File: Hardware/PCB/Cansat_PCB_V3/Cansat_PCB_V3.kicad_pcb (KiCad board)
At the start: 6 copper layers, 33.6 x 25.4 mm, 100 parts, among them IC1 Alim STM Baro GPS IMU, IC2 Alim LoRa, J1 Lecteur SD, J10 Connecteur IHM, J2 Connecteur Batterie, J3 Connecteur STLINK, J4 Connecteur Moteur, J5 Connecteur TOF, J6 Connecteur GPS, J7 Connecteur LoRa, J9 Connecteur Camera, SW1 RSTBTN, SW2 boot, U1 Barometre BMP581, U2 STM32G431CBUx, U3 IMU BNO055, U5 LMR51625, Y1 Crystal_GND24_Small, Y2 Oscillateur_IMU

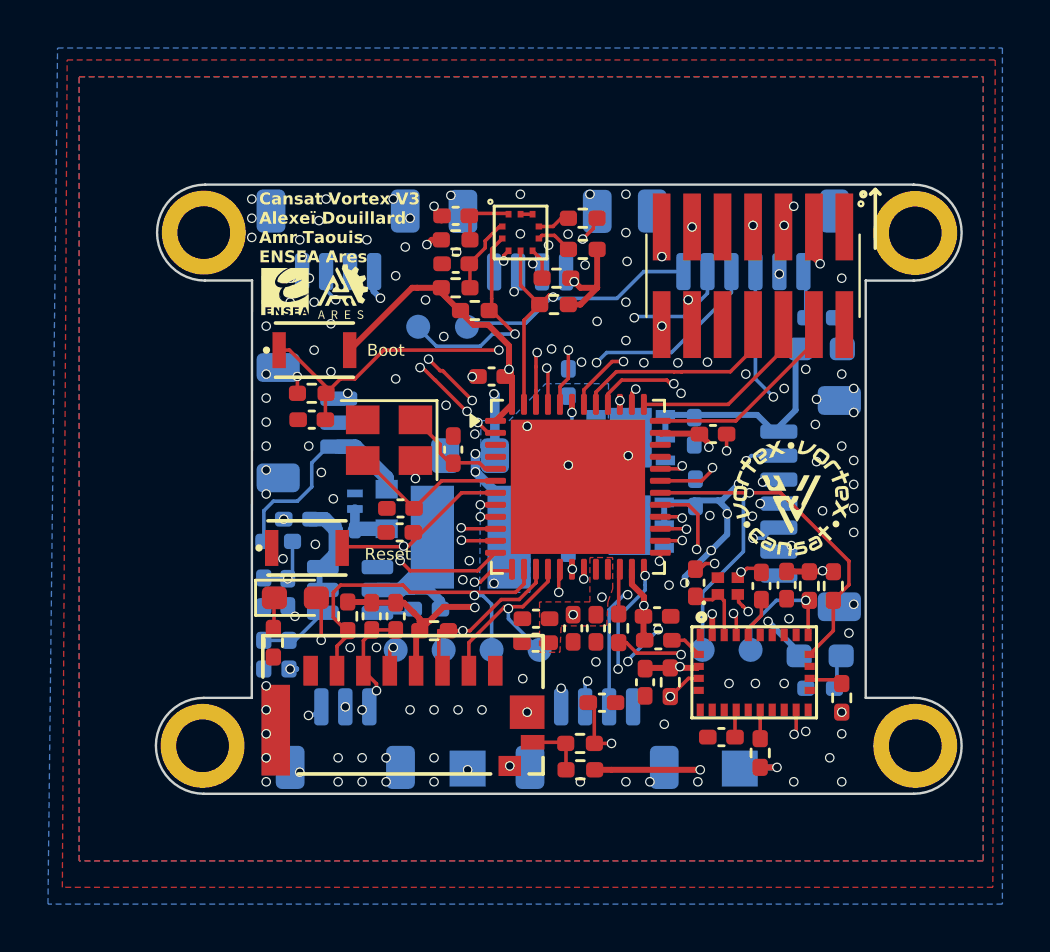
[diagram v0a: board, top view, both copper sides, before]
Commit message: mega big readme update for the mechanical and wind tunnel parts
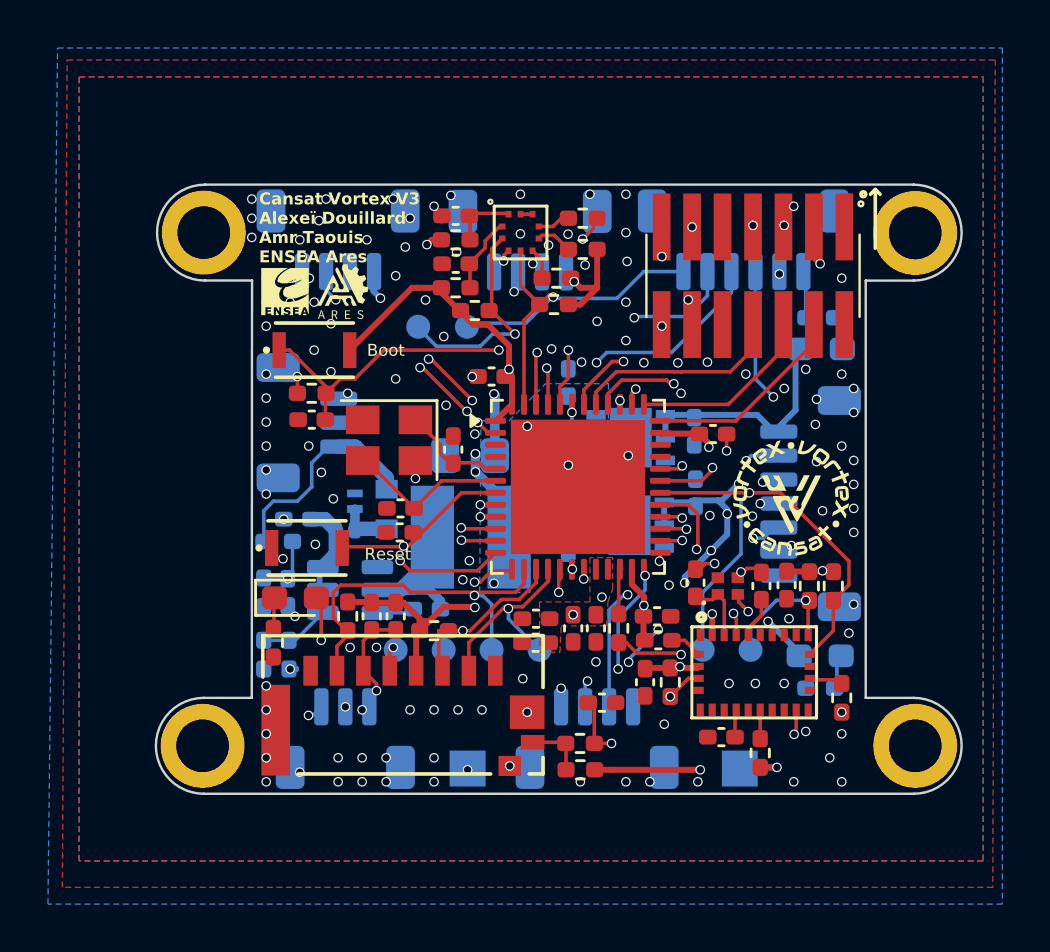
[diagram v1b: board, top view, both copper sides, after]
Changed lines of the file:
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@@
 			(drillshape 0)
 			(scaleselection 1)
-			(outputdirectory "/home/alexei/Bureau/Gerber_Cansat/")
+			(outputdirectory "/home/alexei/Bureau/Gerber_Cansat_V3/")
 		)
 	)
@@
 	)
 	(segment
-		(start 144.356471 95.85646)
-		(end 144.4 95.899989)
-		(width 0.15)
-		(layer "F.Cu")
-		(net 24)
-	)
-	(segment
-		(start 145.59 97.09)
-		(end 145.59 97.1)
+		(start 143.7716 95.375)
+		(end 143.875011 95.375)
 		(width 0.15)
 		(layer "F.Cu")
@@
 	)
 	(segment
-		(start 144.25306 95.85646)
-		(end 144.356471 95.85646)
+		(start 144.4 95.9)
+		(end 145.59 97.09)
 		(width 0.15)
 		(layer "F.Cu")
@@
 	)
 	(segment
-		(start 143.7716 95.375)
-		(end 144.25306 95.85646)
+		(start 143.875011 95.375)
+		(end 144.4 95.899989)
 		(width 0.15)
 		(layer "F.Cu")
@@
 	)
 	(segment
-		(start 144.4 95.9)
-		(end 145.59 97.09)
+		(start 144.4 95.899989)
+		(end 144.4 95.9)
 		(width 0.15)
 		(layer "F.Cu")
@@
 	)
 	(segment
-		(start 144.4 95.899989)
-		(end 144.4 95.9)
+		(start 145.59 97.09)
+		(end 145.59 97.1)
 		(width 0.15)
 		(layer "F.Cu")
@@
 	)
 	(segment
-		(start 143.4154 95.7278)
-		(end 143.520693 95.7278)
+		(start 143.520693 95.7278)
+		(end 145.344534 97.551641)
 		(width 0.15)
 		(layer "F.Cu")
@@
 	)
 	(segment
-		(start 144.059956 96.259956)
-		(end 145.351641 97.551641)
-		(width 0.15)
-		(layer "F.Cu")
-		(net 25)
-	)
-	(segment
 		(start 149.25 96.525)
 		(end 149.25 97.2625)
@@
 	)
 	(segment
-		(start 144.052849 96.259956)
-		(end 144.059956 96.259956)
+		(start 149.6 95)
+		(end 149.6 96.175)
 		(width 0.15)
 		(layer "F.Cu")
@@
 	)
 	(segment
-		(start 145.351641 97.551641)
+		(start 145.344534 97.551641)
 		(end 145.37547 97.551641)
 		(width 0.15)
@@
 	)
 	(segment
-		(start 149.6 95)
-		(end 149.6 96.175)
+		(start 143.4154 95.7278)
+		(end 143.520693 95.7278)
 		(width 0.15)
 		(layer "F.Cu")
@@
 		(net 25)
 	)
-	(segment
-		(start 143.520693 95.7278)
-		(end 144.052849 96.259956)
-		(width 0.15)
-		(layer "F.Cu")
-		(net 25)
-	)
 	(via
 		(at 149.6 95)
@@
 	)
 	(segment
-		(start 155.4 92.630043)
+		(start 155.4 92.7348)
 		(end 155.4 91.825)
 		(width 0.15)
@@
 	)
 	(segment
-		(start 154.430043 93.6)
-		(end 155.4 92.630043)
+		(start 154.5348 93.6)
+		(end 155.4 92.7348)
 		(width 0.15)
 		(layer "B.Cu")
@@
 	)
 	(segment
-		(start 152.35 93.65)
-		(end 152.4 93.6)
+		(start 147.375 94.330262)
+		(end 146.438538 94.330262)
 		(width 0.15)
 		(layer "B.Cu")
@@
 	)
 	(segment
-		(start 147.375 94.330262)
-		(end 146.438538 94.330262)
+		(start 152.4 93.6)
+		(end 154.5348 93.6)
 		(width 0.15)
 		(layer "B.Cu")
@@
 	)
 	(segment
-		(start 152.4 93.6)
-		(end 154.430043 93.6)
+		(start 152.35 93.65)
+		(end 152.4 93.6)
 		(width 0.15)
 		(layer "B.Cu")
@@
 	)
 	(via
-		(at 152.084834 107.984834)
+		(at 152.112507 108.011093)
 		(size 0.4)
 		(drill 0.3)
@@
 	)
 	(segment
-		(start 152.084834 107.922835)
-		(end 153.35 106.657669)
+		(start 152.084834 107.98342)
+		(end 152.084834 107.922835)
 		(width 0.15)
 		(layer "B.Cu")
@@
 	)
 	(segment
-		(start 152.084834 107.984834)
-		(end 152.084834 107.922835)
+		(start 152.084834 107.922835)
+		(end 153.35 106.657669)
 		(width 0.15)
 		(layer "B.Cu")
@@
 	)
 	(segment
-		(start 138.764589 110.232295)
-		(end 138.942705 110.232295)
+		(start 152.112507 108.011093)
+		(end 152.084834 107.98342)
 		(width 0.15)
 		(layer "B.Cu")
@@
 	)
 	(segment
-		(start 138.764589 110.419557)
-		(end 139.721808 111.376776)
+		(start 138.764589 110.232295)
+		(end 138.942705 110.232295)
 		(width 0.15)
-		(layer "In2.Cu")
+		(layer "B.Cu")
 		(net 41)
 	)
 	(segment
-		(start 152.084834 108.615166)
-		(end 152.084834 107.984834)
+		(start 154.95 103.310799)
+		(end 154.95 103.45)
 		(width 0.15)
 		(layer "In2.Cu")
@@
 	)
 	(segment
-		(start 154.95 103.310799)
-		(end 154.95 103.45)
+		(start 139.721808 111.376776)
+		(end 138.764589 110.419557)
 		(width 0.15)
 		(layer "In2.Cu")
@@
 	)
 	(segment
-		(start 138.764589 110.232295)
-		(end 138.764589 110.419557)
+		(start 149.323224 111.376776)
+		(end 139.721808 111.376776)
 		(width 0.15)
 		(layer "In2.Cu")
@@
 	)
 	(segment
-		(start 139.721808 111.376776)
-		(end 149.323224 111.376776)
+		(start 138.764589 110.419557)
+		(end 138.764589 110.232295)
 		(width 0.15)
 		(layer "In2.Cu")
@@
 	)
 	(segment
-		(start 149.323224 111.376776)
+		(start 152.084834 108.615166)
+		(end 149.323224 111.376776)
+		(width 0.15)
+		(layer "In2.Cu")
+		(net 41)
+	)
+	(segment
+		(start 152.084834 108.038766)
 		(end 152.084834 108.615166)
 		(width 0.15)
@@
 	)
 	(segment
+		(start 152.112507 108.011093)
+		(end 152.084834 108.038766)
+		(width 0.15)
+		(layer "In2.Cu")
+		(net 41)
+	)
+	(segment
 		(start 152.8 104.1875)
 		(end 152.75 104.1375)
@@
 	(segment
 		(start 157.15 100.95)
-		(end 156.9 101.2)
+		(end 156.8012 101.2988)
 		(width 0.15)
 		(layer "B.Cu")
@@
 	)
 	(segment
-		(start 155.2 105.1)
-		(end 155.2 107.5)
+		(start 156.8012 103.4988)
+		(end 155.2 105.1)
 		(width 0.15)
 		(layer "B.Cu")
@@
 	)
 	(segment
-		(start 156.9 101.2)
-		(end 156.9 103.4)
+		(start 155.2 105.1)
+		(end 155.2 107.5)
 		(width 0.15)
 		(layer "B.Cu")
@@
 	)
 	(segment
-		(start 156.9 103.4)
-		(end 155.2 105.1)
+		(start 156.8012 101.2988)
+		(end 156.8012 103.4988)
 		(width 0.15)
 		(layer "B.Cu")
